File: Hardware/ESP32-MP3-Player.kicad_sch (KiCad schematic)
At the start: 17 parts, among them J1 Micro_SD_Card, J2 AudioJack3, J3 Battery, SW1 Reset, U1 ESP32-WROOM-32E, U2 MAX98357A, U3 AMS1117-3.3

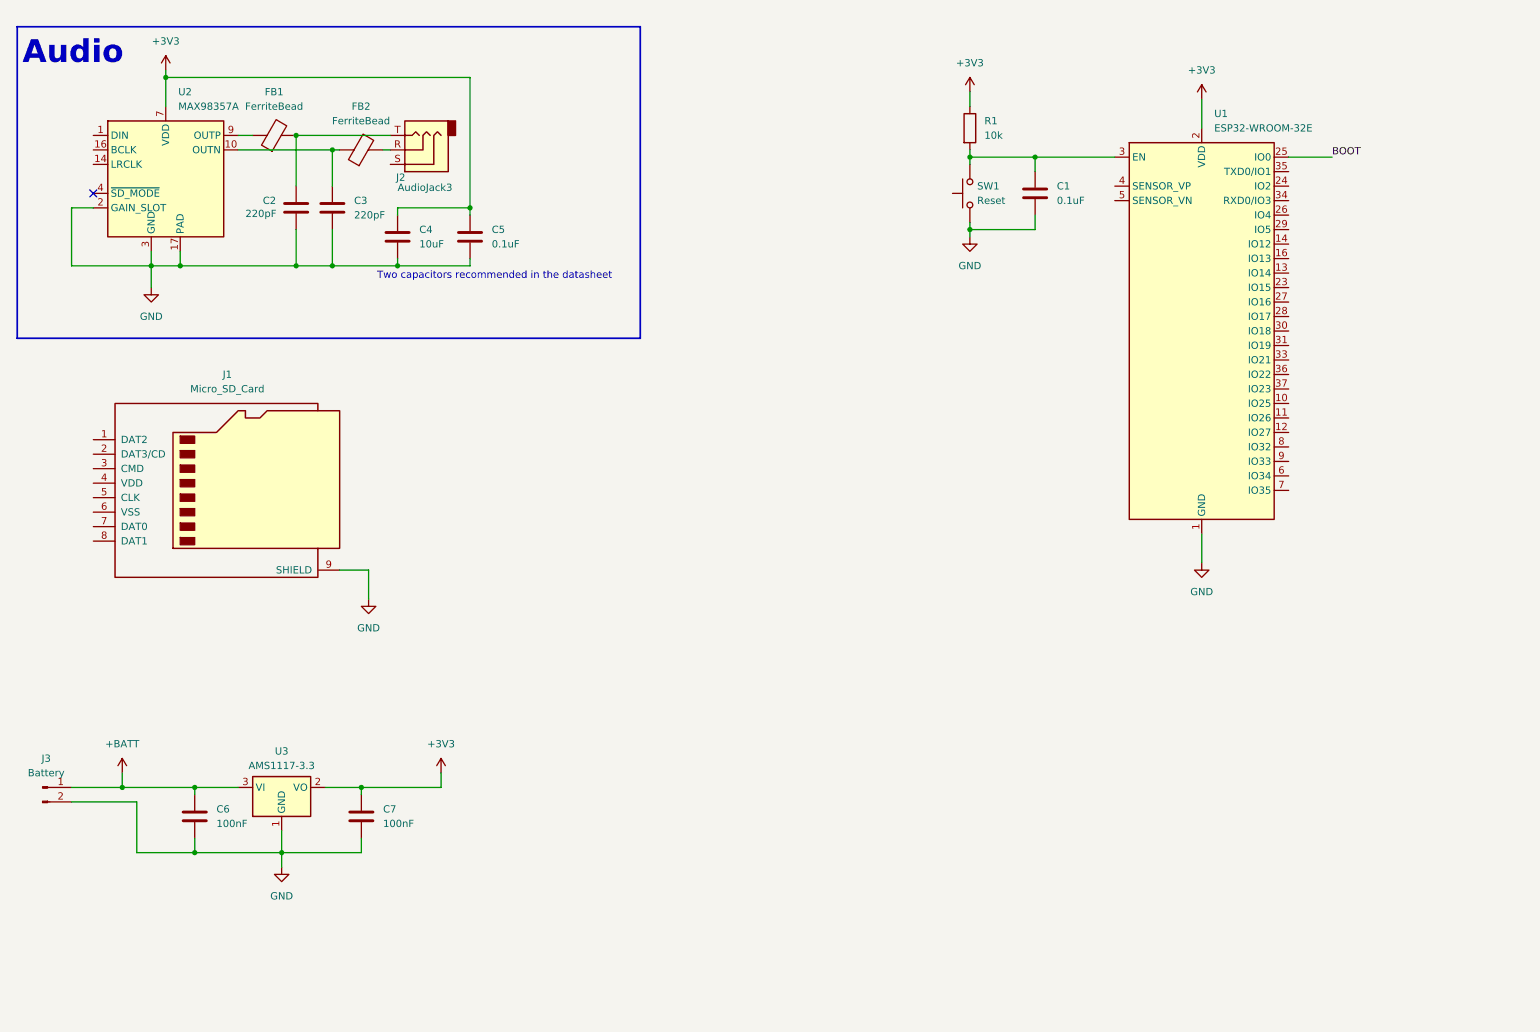
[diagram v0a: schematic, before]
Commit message: hardware: new analog circuit design
The old username is deprecated
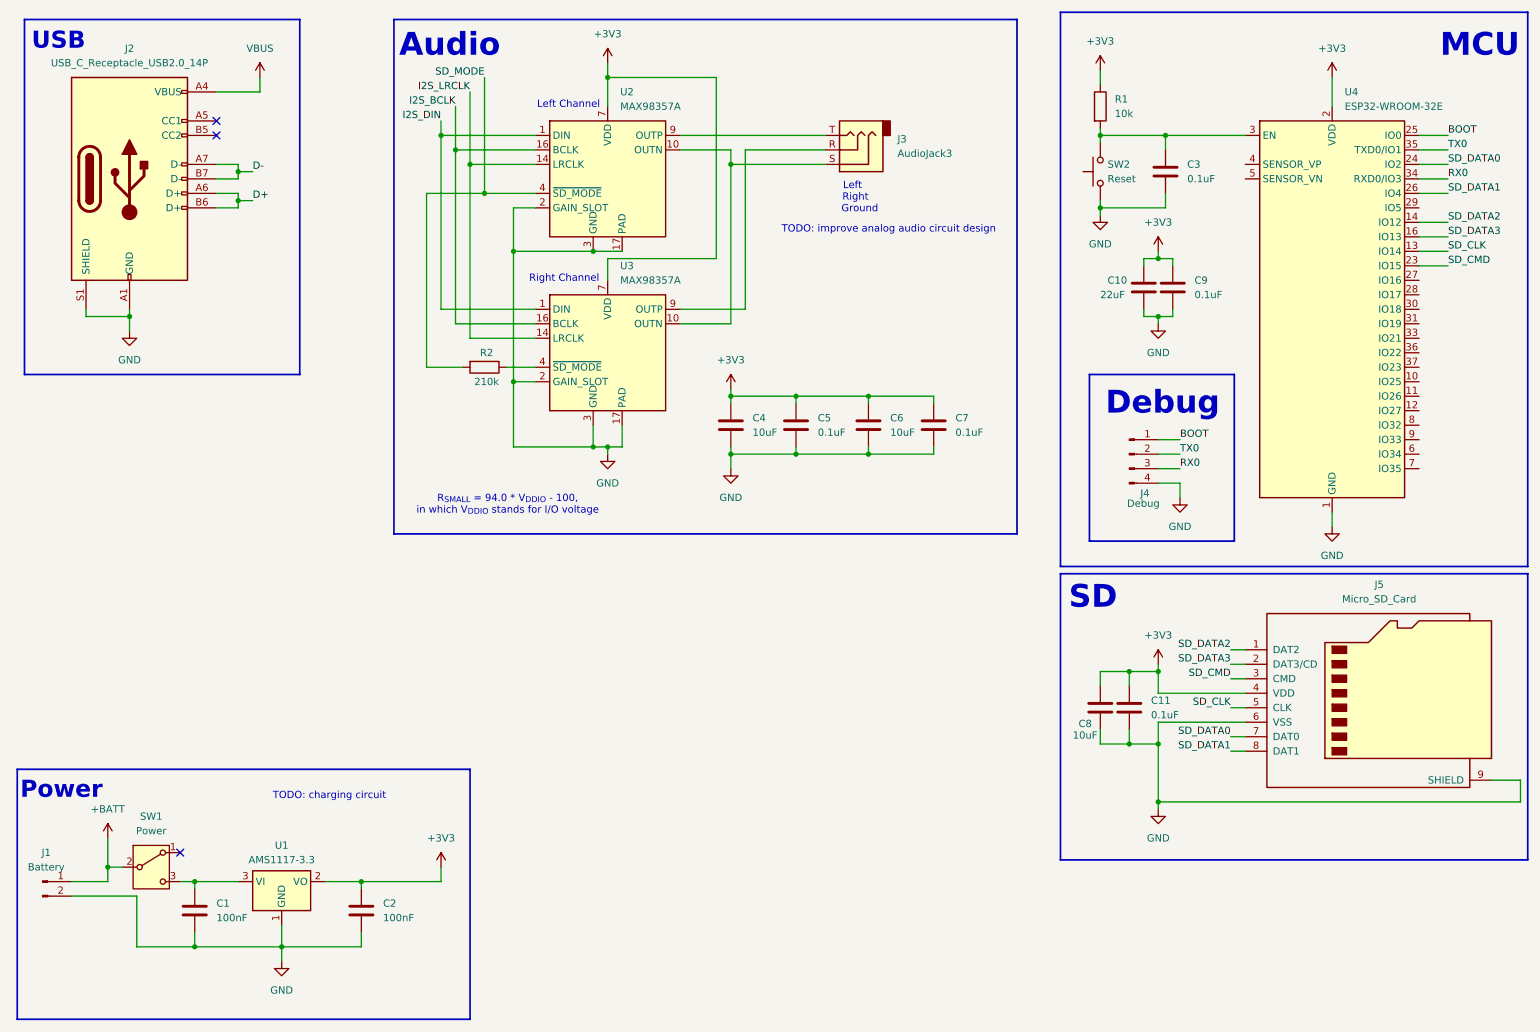
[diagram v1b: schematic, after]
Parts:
- removed C2, C3: 220pF, symbol Device:C
- removed FB1, FB2: FerriteBead, symbol Device:FerriteBead
- removed J2: AudioJack3, symbol Connector_Audio:AudioJack3
- added C10: 22uF, symbol Device:C
- added C11, C7, C9: 0.1uF, symbol Device:C
- added C6, C8: 10uF, symbol Device:C
- added J2: USB_C_Receptacle_USB2.0_14P, symbol Connector:USB_C_Receptacle_USB2.0_14P
- added J3: AudioJack3, symbol Connector_Audio:AudioJack3
- added J4: Debug, symbol Connector:Conn_01x04_Pin
- added R2: 210k, symbol Device:R
- added SW1: Power, symbol Switch:SW_SPDT
- added U3: MAX98357A, Package_DFN_QFN:TQFN-16-1EP_3x3mm_P0.5mm_EP1.23x1.23mm, symbol Audio:MAX98357A
- renumbered C6 to C1, C7 to C2, C1 to C3, J3 to J1, J1 to J5, SW1 to SW2, U3 to U1, U1 to U4
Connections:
- net +3V3: now also J5.4 (VDD), C10.1, C11.1, C6.1, C7.1, C8.1, C9.1, U3.7 (VDD), U3.8 (VDD)
- net +BATT: now also SW1.2 (B); no longer C1.1, U1.3 (VI)
- net BOOT: now also J4.1 (Pin_1)
- net GND: now also J5.6 (VSS), C10.2, C11.2, C6.2, C7.2, C8.2, C9.2, J2.A1 (GND), J2.A12 (GND), J2.B1 (GND), J2.B12 (GND), J2.S1 (SHIELD), J4.4 (Pin_4), U3.11 (GND), U3.15 (GND), U3.17 (PAD), U3.2 (GAIN_SLOT), U3.3 (GND)
- net at U2.9 (OUTP): now also J3.T
- net SD_DATA2: now reaches J5.1 (DAT2)
- net SD_DATA2: now also U4.14 (IO12)
- net SD_DATA3: now reaches J5.2 (DAT3/CD)
- net SD_DATA3: now also U4.16 (IO13)
- net SD_CMD: now reaches J5.3 (CMD)
- net SD_CMD: now also U4.23 (IO15)
- net SD_CLK: now reaches J5.5 (CLK)
- net SD_CLK: now also U4.13 (IO14)
- net SD_DATA0: now reaches J5.7 (DAT0)
- net SD_DATA0: now also U4.24 (IO2)
- net SD_DATA1: now reaches J5.8 (DAT1)
- net SD_DATA1: now also U4.26 (IO4)
- net at U2.10 (OUTN): now also J3.S, U3.10 (OUTN)
- net I2S_DIN: now reaches U2.1 (DIN)
- net I2S_DIN: now also U3.1 (DIN)
- net I2S_LRCLK: now reaches U2.14 (LRCLK)
- net I2S_LRCLK: now also U3.14 (LRCLK)
- net I2S_BCLK: now reaches U2.16 (BCLK)
- net I2S_BCLK: now also U3.16 (BCLK)
- net SD_MODE: now reaches U2.4 (~{SD_MODE})
- net SD_MODE: now also R2.2
- net RX0: now reaches U4.34 (RXD0/IO3)
- net RX0: now also J4.3 (Pin_3)
- net TX0: now reaches U4.35 (TXD0/IO1)
- net TX0: now also J4.2 (Pin_2)
- new net: J3.R, U3.9 (OUTP)
- new net: R2.1, U3.4 (~{SD_MODE})
- new net: C1.1, SW1.3 (C), U1.3 (VI)
- new net D+: J2.A6 (D+), J2.B6 (D+)
- new net D-: J2.A7 (D-), J2.B7 (D-)
- new net VBUS: J2.A4 (VBUS), J2.A9 (VBUS), J2.B4 (VBUS), J2.B9 (VBUS)
- no-connect marks 1 -> 3
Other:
- note added: "Debug"
- note added: "Ground"
- note added: "Left"
- note added: "Left Channel"
- note added: "MCU"
- note added: "Power"
- note added: "R_{SMALL} = 94.0 * V_{DDIO} - 100, in which V_{DDIO} stands for I/O voltage"
- note added: "Right"
- note added: "Right Channel"
- note added: "SD"
- note added: "TODO: charging circuit"
- note added: "TODO: improve analog audio circuit design"
- note added: "USB"
- note removed: "Two capacitors recommended in the datasheet"
- company: (none) -> Chubbyginger
- title: (none) -> ESP32-MP3-Player
- moved on the sheet: C1, C2, C3, J1, J5, R1, SW2, U1, U4
